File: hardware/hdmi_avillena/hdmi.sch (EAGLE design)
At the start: 10 parts

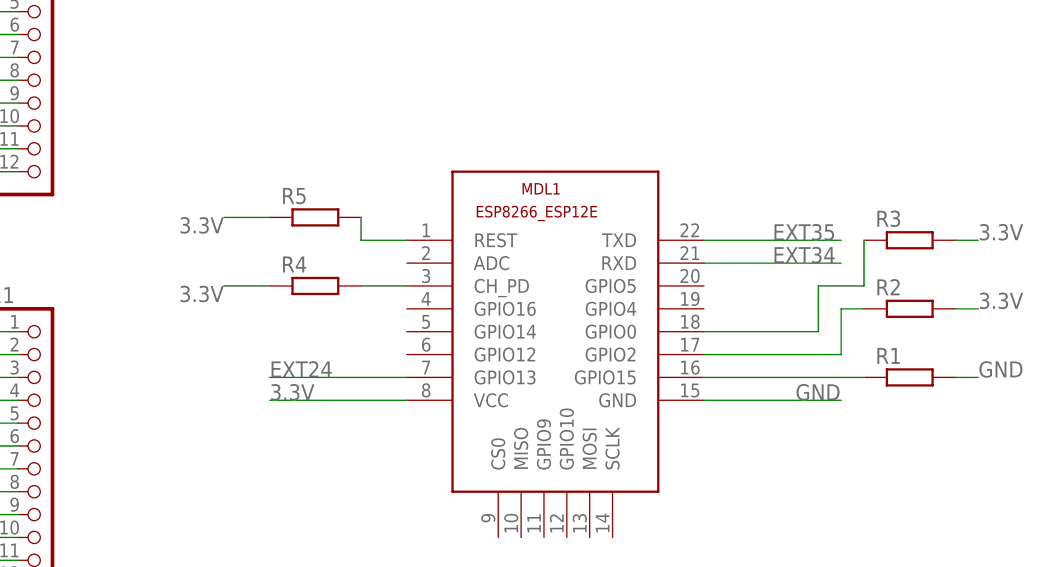
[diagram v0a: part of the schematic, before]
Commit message: Últimas correcciones de yombo
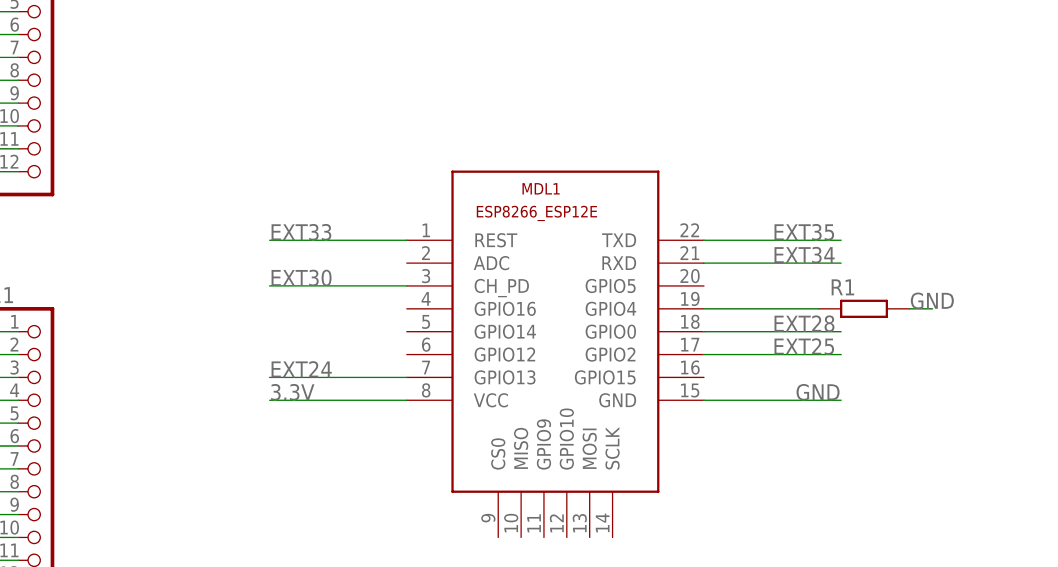
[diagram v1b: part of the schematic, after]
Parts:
- removed R2, R3, R4, R5: (no value), rcl:R-EU_M0805
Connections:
- removed net N$2: MDL1.GPIO15, R1.1
- removed net N$3: MDL1.GPIO2, R2.1
- removed net N$4: MDL1.GPIO0, R3.1
- removed net N$5: MDL1.REST, R5.2
- net 3.3V: no longer R2.2, R3.2, R4.1, R5.1
- net EXT25: now also MDL1.GPIO2
- net EXT28: now also MDL1.GPIO0
- net EXT30: now also MDL1.CH_PD
- net EXT33: now also MDL1.REST
- net N$1: now also MDL1.GPIO4, R1.1; no longer MDL1.CH_PD, R4.2
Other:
- moved on the sheet: R1
